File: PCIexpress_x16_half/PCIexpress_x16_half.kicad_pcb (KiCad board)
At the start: 4 copper layers, 167.7 x 111.2 mm, 66 parts, among them J1 PCIexpress_bracket, J2 PCIexpress_x16

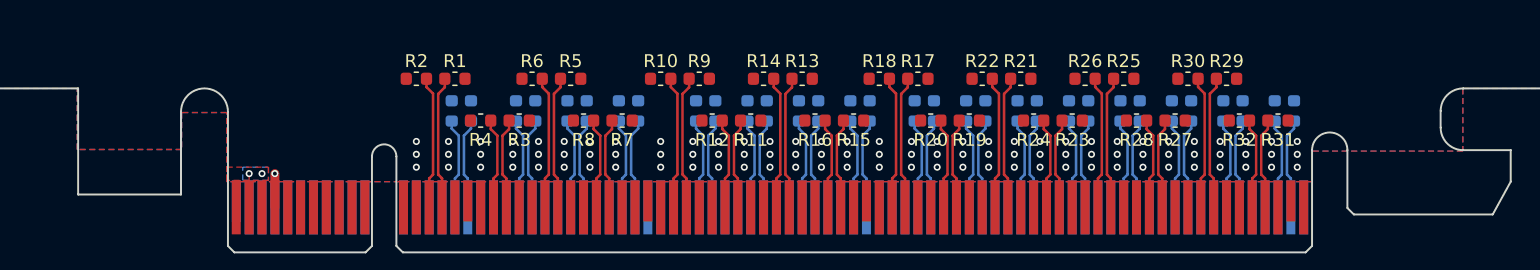
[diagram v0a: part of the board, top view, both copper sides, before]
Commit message: templates
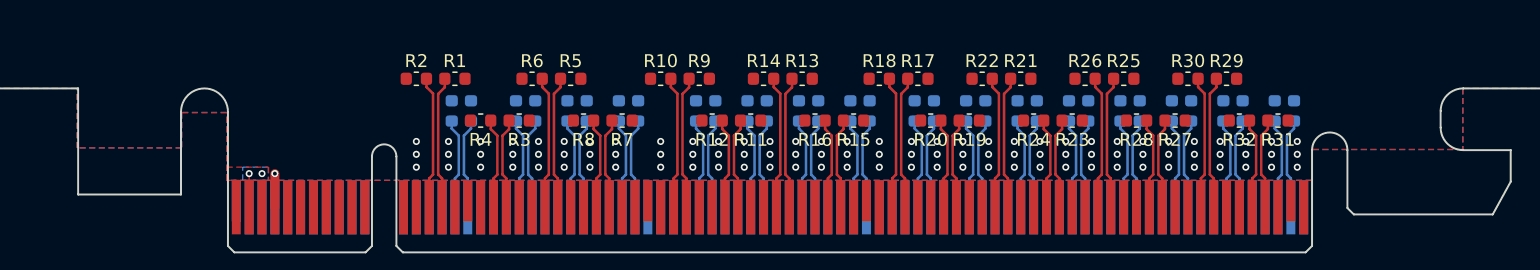
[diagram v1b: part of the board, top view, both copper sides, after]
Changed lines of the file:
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@@
-(kicad_pcb (version 20171130) (host pcbnew 5.1.2-f72e74a~84~ubuntu16.04.1)
+(kicad_pcb (version 20171130) (host pcbnew 5.1.3-ffb9f22~84~ubuntu16.04.1)
   (general
     (thickness 1.6)
-    (drawings 51)
+    (drawings 52)
     (tracks 425)
     (zones 0)
@@
     (pad_to_mask_clearance 0.051)
     (solder_mask_min_width 0.25)
-    (aux_axis_origin 0 0)
-    (grid_origin 109.375 194.125)
+    (aux_axis_origin 109.625 194.125)
+    (grid_origin 109.625 194.125)
     (visible_elements FFFDFFFF)
     (pcbplotparams
@@
     )
   )
+  (target plus (at 109.625 194.125) (size 5) (width 0.05) (layer Edge.Cuts))
   (gr_line (start 232.1277 181.375) (end 205.525 181.375) (layer Edge.Cuts) (width 0.15))
   (gr_line (start 232.125 82.975) (end 232.1277 181.375) (layer Edge.Cuts) (width 0.15))
@@
     (polygon
       (pts
-        (xy 64.5 83) (xy 232.125 83) (xy 232.125 181.375) (xy 205.5 181.375) (xy 205.5 186.25)
-        (xy 193.75 186.25) (xy 193.75 188.625) (xy 109.375 188.625) (xy 109.375 183.25) (xy 105.875 183.25)
-        (xy 105.875 186.125) (xy 97.75 186.125) (xy 97.75 181.375) (xy 79.5 181.375) (xy 79.5 189.625)
+        (xy 64.5 83) (xy 232.125 83) (xy 232.125 181.375) (xy 205.5 181.375) (xy 205.5 186.125)
+        (xy 193.75 186.125) (xy 193.75 188.525) (xy 109.375 188.525) (xy 109.375 183.25) (xy 105.875 183.25)
+        (xy 105.875 186) (xy 97.75 186) (xy 97.75 181.375) (xy 79.5 181.375) (xy 79.5 189.625)
         (xy 64.5 189.625)
       )
@@
     (polygon
       (pts
-        (xy 64.5 83) (xy 232.125 83) (xy 232.125 181.375) (xy 205.5 181.375) (xy 205.5 186.25)
-        (xy 193.75 186.25) (xy 193.75 188.625) (xy 109.375 188.625) (xy 109.375 183.25) (xy 105.875 183.25)
-        (xy 105.875 186.125) (xy 97.75 186.125) (xy 97.75 181.375) (xy 79.5 181.375) (xy 79.5 189.625)
+        (xy 64.5 83) (xy 232.125 83) (xy 232.125 181.375) (xy 205.5 181.375) (xy 205.5 186.125)
+        (xy 193.75 186.125) (xy 193.75 188.525) (xy 109.375 188.525) (xy 109.375 183.25) (xy 105.875 183.25)
+        (xy 105.875 186) (xy 97.75 186) (xy 97.75 181.375) (xy 79.5 181.375) (xy 79.5 189.625)
         (xy 64.5 189.625)
       )
@@
     (polygon
       (pts
-        (xy 64.5 83) (xy 232.125 83) (xy 232.125 181.375) (xy 205.5 181.375) (xy 205.5 186.25)
-        (xy 193.75 186.25) (xy 193.75 188.625) (xy 109.375 188.625) (xy 109.375 183.25) (xy 105.875 183.25)
-        (xy 105.875 186.125) (xy 97.75 186.125) (xy 97.75 181.375) (xy 79.5 181.375) (xy 79.5 189.625)
+        (xy 64.5 83) (xy 232.125 83) (xy 232.125 181.375) (xy 205.5 181.375) (xy 205.5 186.125)
+        (xy 193.75 186.125) (xy 193.75 188.525) (xy 109.375 188.525) (xy 109.375 183.25) (xy 105.875 183.25)
+        (xy 105.875 186) (xy 97.75 186) (xy 97.75 181.375) (xy 79.5 181.375) (xy 79.5 189.625)
         (xy 64.5 189.625)
       )
@@
     (polygon
       (pts
-        (xy 64.5 83) (xy 232.125 83) (xy 232.125 181.375) (xy 205.5 181.375) (xy 205.5 186.25)
-        (xy 193.75 186.25) (xy 193.75 188.625) (xy 109.375 188.625) (xy 109.375 183.25) (xy 105.875 183.25)
-        (xy 105.875 186.125) (xy 97.75 186.125) (xy 97.75 181.375) (xy 79.5 181.375) (xy 79.5 189.625)
+        (xy 64.5 83) (xy 232.125 83) (xy 232.125 181.375) (xy 205.5 181.375) (xy 205.5 186.125)
+        (xy 193.75 186.125) (xy 193.75 188.525) (xy 109.375 188.525) (xy 109.375 183.25) (xy 105.875 183.25)
+        (xy 105.875 186) (xy 97.75 186) (xy 97.75 181.375) (xy 79.5 181.375) (xy 79.5 189.625)
         (xy 64.5 189.625)
       )

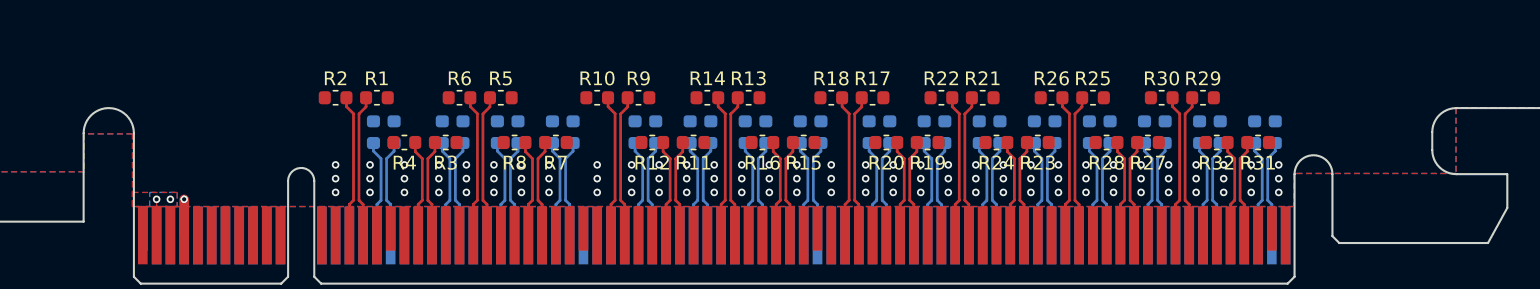
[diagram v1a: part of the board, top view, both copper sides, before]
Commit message: KiCad 6 update
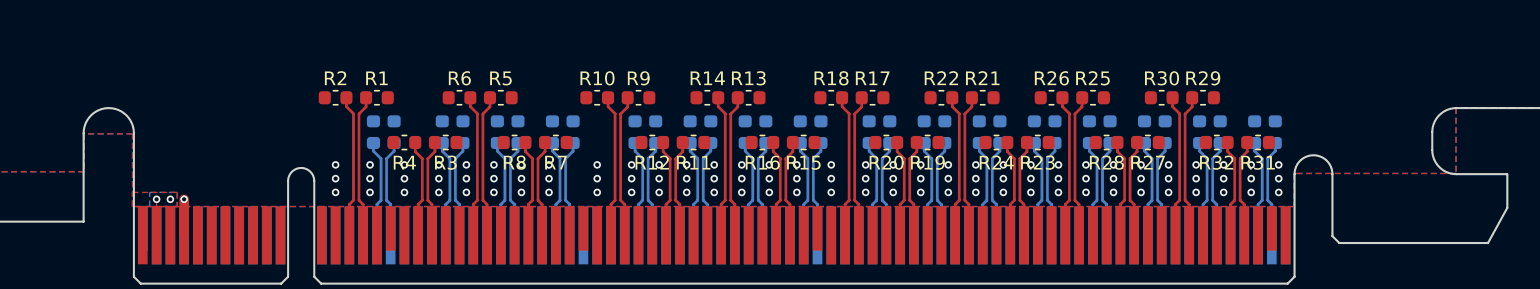
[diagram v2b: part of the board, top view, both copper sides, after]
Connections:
- net /~PERST renamed /~{PERST}
- net /~PRSNT1 renamed /~{PRSNT1}
- net /~PRSNT2x1 renamed /~{PRSNT2x1}
- net /~PRSNT2x16 renamed /~{PRSNT2x16}
- net /~PRSNT2x4 renamed /~{PRSNT2x4}
- net /~PRSNT2x8 renamed /~{PRSNT2x8}
- net /~TRST renamed /~{TRST}
- net /~WAKE renamed /~{WAKE}
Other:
- net class Default removed
- net class Diff-100-PCIe removed
- net class JLC2313-100d-3.5 removed
- net class JLC2313-100d-4 removed
- net class JLC7628-100d-8 removed
